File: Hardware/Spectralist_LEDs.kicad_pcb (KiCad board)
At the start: 2 copper layers, 40 x 37 mm, 34 parts, among them J1 Conn_01x03_Pin, J2 Conn_01x02_Pin, J3 Conn_01x02_Pin, U1 PCA9956B_LED_Driver

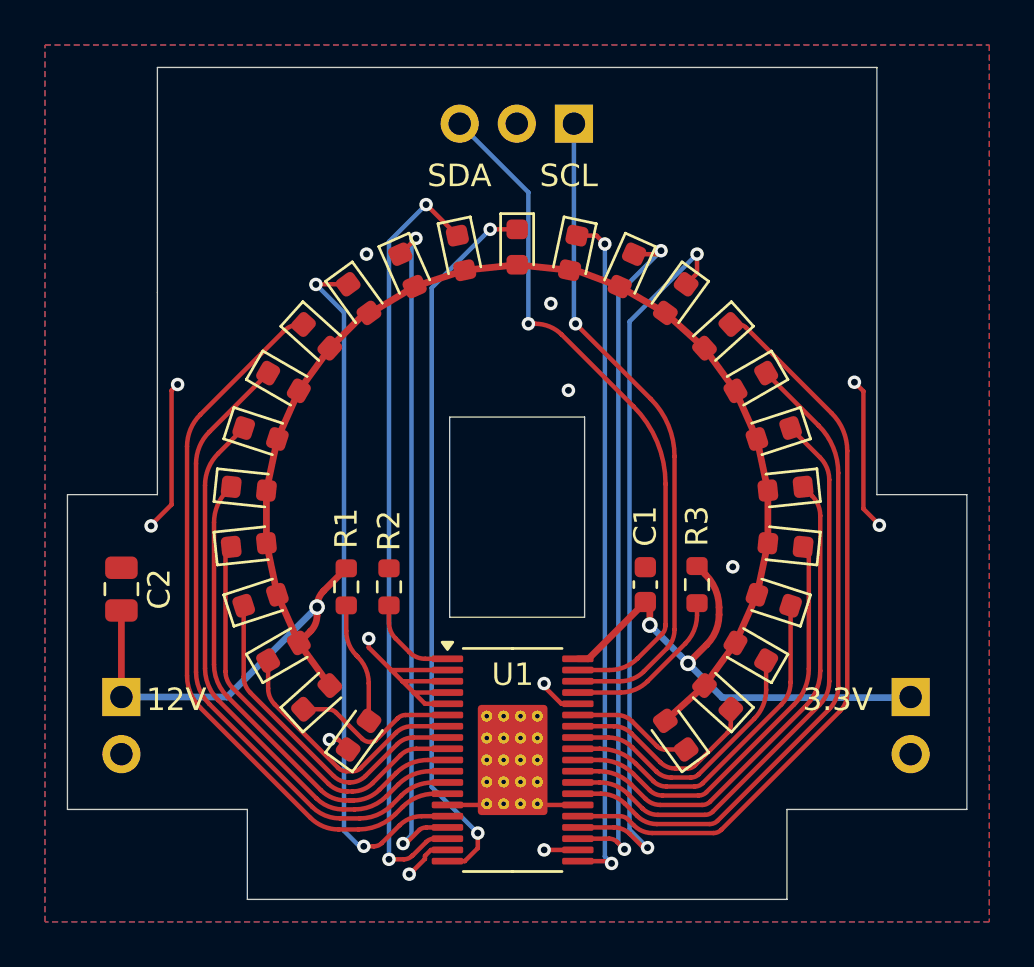
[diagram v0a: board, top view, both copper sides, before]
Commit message: v1.0 PCBs sent to production
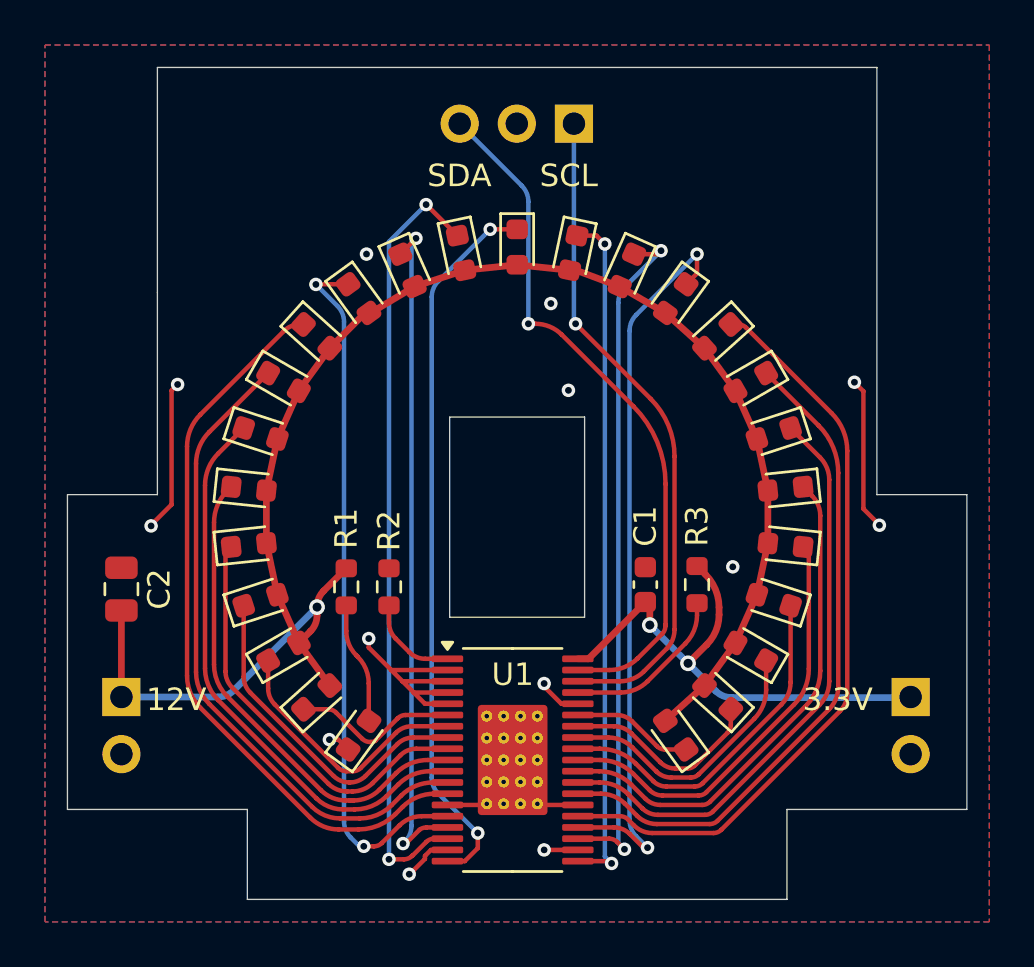
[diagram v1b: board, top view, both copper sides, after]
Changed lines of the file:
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@@
 			(outputformat 1)
 			(mirror no)
-			(drillshape 1)
+			(drillshape 0)
 			(scaleselection 1)
-			(outputdirectory "")
+			(outputdirectory "Gerbers/Spectralist_LEDs")
 		)
 	)
@@
 		)
 	)
+	(gr_text_box "Mountjoy Modular 2025\nSpectralist LEDs v1.0\n"
+		(start 140.45 83.1)
+		(end 144.75 103.4)
+		(angle 90)
+		(layer "B.SilkS")
+		(effects
+			(font
+				(size 1 1)
+				(thickness 0.1)
+			)
+			(justify top mirror)
+		)
+		(border yes)
+		(stroke
+			(width 0.1)
+			(type solid)
+		)
+	)
 	(segment
 		(start 125.22038 117.87962)
@@
 	(segment
 		(start 121.1 106)
-		(end 117.1 110)
+		(end 117.392893 109.707107)
 		(width 0.3)
 		(layer "B.Cu")
@@
 	)
 	(segment
-		(start 117.1 110)
+		(start 116.685786 110)
 		(end 112.4 110)
 		(width 0.3)
@@
 		(net 2)
 	)
+	(arc
+		(start 116.685786 110)
+		(mid 117.068469 109.92388)
+		(end 117.392893 109.707107)
+		(width 0.3)
+		(layer "B.Cu")
+		(net 2)
+	)
 	(segment
 		(start 123.461136 112)
@@
 	)
 	(segment
-		(start 122.3 115.95)
-		(end 122.3 92.9)
+		(start 122.3 115.535786)
+		(end 122.3 93.314214)
 		(width 0.2)
 		(layer "B.Cu")
@@
 	)
 	(segment
-		(start 122.3 92.9)
+		(start 122.007107 92.607107)
 		(end 121.05 91.65)
 		(width 0.2)
@@
 	(segment
 		(start 122.99 116.64)
-		(end 122.3 115.95)
+		(end 122.592893 116.242893)
+		(width 0.2)
+		(layer "B.Cu")
+		(net 11)
+	)
+	(arc
+		(start 122.007107 92.607107)
+		(mid 122.22388 92.93153)
+		(end 122.3 93.314214)
+		(width 0.2)
+		(layer "B.Cu")
+		(net 11)
+	)
+	(arc
+		(start 122.592893 116.242893)
+		(mid 122.37612 115.91847)
+		(end 122.3 115.535786)
 		(width 0.2)
 		(layer "B.Cu")
@@
 	)
 	(segment
-		(start 125.3 116.140915)
+		(start 125.007107 116.433808)
 		(end 124.923586 116.517329)
 		(width 0.2)
@@
 	(segment
 		(start 125.3 89.799996)
-		(end 125.3 116.140915)
+		(end 125.3 115.726701)
+		(width 0.2)
+		(layer "B.Cu")
+		(net 12)
+	)
+	(arc
+		(start 125.3 115.726701)
+		(mid 125.22388 116.109384)
+		(end 125.007107 116.433808)
 		(width 0.2)
 		(layer "B.Cu")
@@
 	)
 	(segment
-		(start 126.2 91.799998)
+		(start 126.492893 91.507105)
 		(end 128.8 89.199998)
 		(width 0.2)
@@
 	(segment
 		(start 128.25 116.05)
-		(end 126.2 114)
+		(end 126.492893 114.292893)
 		(width 0.2)
 		(layer "B.Cu")
@@
 	)
 	(segment
-		(start 126.2 114)
-		(end 126.2 91.799998)
+		(start 126.2 113.585786)
+		(end 126.2 92.214212)
+		(width 0.2)
+		(layer "B.Cu")
+		(net 14)
+	)
+	(arc
+		(start 126.492893 91.507105)
+		(mid 126.27612 91.831528)
+		(end 126.2 92.214212)
+		(width 0.2)
+		(layer "B.Cu")
+		(net 14)
+	)
+	(arc
+		(start 126.2 113.585786)
+		(mid 126.27612 113.968469)
+		(end 126.492893 114.292893)
 		(width 0.2)
 		(layer "B.Cu")
@@
 	(segment
 		(start 136.4 90.15)
-		(end 134.5 92.05)
+		(end 134.792893 91.757107)
 		(width 0.2)
 		(layer "B.Cu")
@@
 	)
 	(segment
-		(start 134.5 92.05)
+		(start 134.5 92.464214)
 		(end 134.5 116.499275)
 		(width 0.2)
@@
 		(net 16)
 	)
+	(arc
+		(start 134.5 92.464214)
+		(mid 134.57612 92.081531)
+		(end 134.792893 91.757107)
+		(width 0.2)
+		(layer "B.Cu")
+		(net 16)
+	)
 	(segment
 		(start 138 91.1585)
@@
 	(segment
 		(start 135.8 116.7)
-		(end 135 115.9)
+		(end 135.292893 116.192893)
 		(width 0.2)
 		(layer "B.Cu")
@@
 	)
 	(segment
-		(start 135 93.3)
+		(start 135.292893 93.007107)
 		(end 138 90.3)
 		(width 0.2)
@@
 	)
 	(segment
-		(start 135 115.9)
-		(end 135 93.3)
+		(start 135 115.485786)
+		(end 135 93.714214)
+		(width 0.2)
+		(layer "B.Cu")
+		(net 17)
+	)
+	(arc
+		(start 135 93.714214)
+		(mid 135.07612 93.331531)
+		(end 135.292893 93.007107)
+		(width 0.2)
+		(layer "B.Cu")
+		(net 17)
+	)
+	(arc
+		(start 135 115.485786)
+		(mid 135.07612 115.868469)
+		(end 135.292893 116.192893)
 		(width 0.2)
 		(layer "B.Cu")
@@
 	(segment
 		(start 130.5 93.4)
-		(end 130.5 87.555)
+		(end 130.5 87.969214)
 		(width 0.2)
 		(layer "B.Cu")
@@
 	)
 	(segment
-		(start 130.5 87.555)
+		(start 130.207107 87.262107)
 		(end 127.445 84.5)
 		(width 0.2)
@@
 		(net 29)
 	)
+	(arc
+		(start 130.5 87.969214)
+		(mid 130.42388 87.586531)
+		(end 130.207107 87.262107)
+		(width 0.2)
+		(layer "B.Cu")
+		(net 29)
+	)
 	(segment
 		(start 132.7 108.3)
@@
 	)
 	(segment
-		(start 139.125 110.025)
+		(start 138.832107 109.732107)
 		(end 135.9 106.8)
 		(width 0.3)
@@
 	(segment
 		(start 147.475 110.025)
-		(end 139.125 110.025)
+		(end 139.539214 110.025)
 		(width 0.3)
 		(layer "B.Cu")
@@
 		(width 0.3)
 		(layer "B.Cu")
+		(net 30)
+	)
+	(arc
+		(start 139.539214 110.025)
+		(mid 139.156531 109.94888)
+		(end 138.832107 109.732107)
+		(width 0.3)
+		(layer "B.Cu")
